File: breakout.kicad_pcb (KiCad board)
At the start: 2 copper layers, 20.7 x 16.1 mm, 7 parts, among them J1 Conn_01x03, J2 Conn_01x02

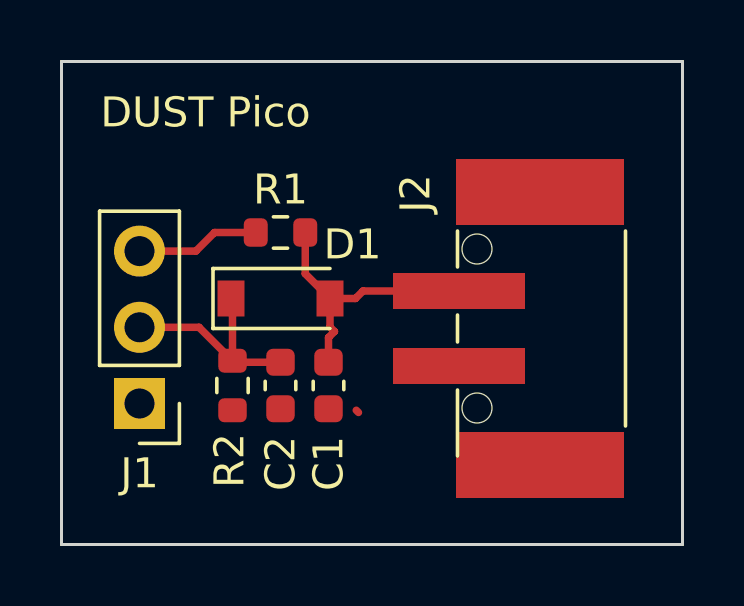
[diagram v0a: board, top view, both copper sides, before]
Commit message: v1.0
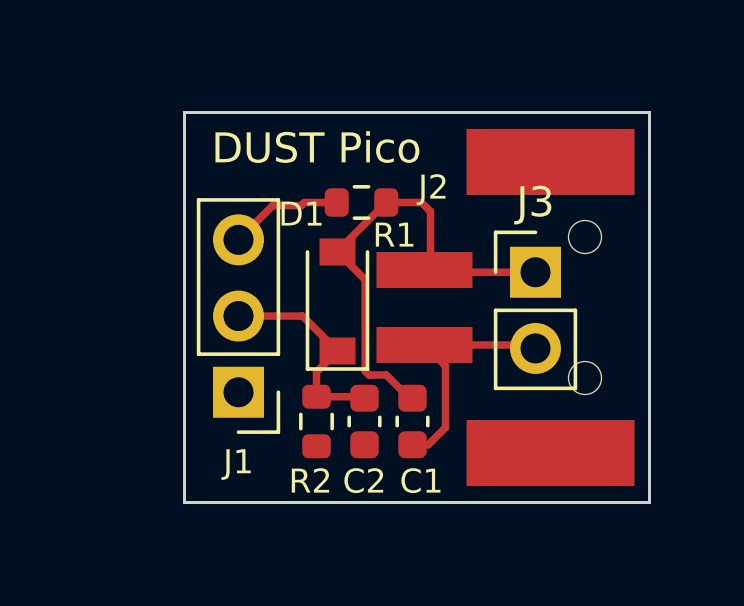
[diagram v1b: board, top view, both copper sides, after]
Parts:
- added J3: Conn_01x02, Connector_PinHeader_2.54mm:PinHeader_1x02_P2.54mm_Vertical, F.Cu at (152.2, 76.3)
- J2: footprint TerminalBlock_Phoenix:TerminalBlock_Phoenix_PTSM-0,5-2-HV-2.5-SMD_1x02-1MP_P2.50mm_Vertical -> DUST:PTSM 0.5-2-HH-2.5-SMD
- moved J1 3.32 mm to (142.3, 80.3)
- moved C2 3.05 mm to (146.5, 81.3)
- moved R2 3.05 mm to (144.9, 81.3)
- moved C1 3.05 mm to (148.1, 81.3)
- moved R1 2.88 mm to (146.4, 74.0)
- moved D1 1.90 mm to (145.6, 77.3), turned to 90 degrees
- moved J2 1.00 mm to (151.6, 77.2), turned to 90 degrees
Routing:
- net Net-(C1-Pad1): track 9.22 -> 16.0 mm
- net GND: track 1.91 -> 8.13 mm
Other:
- board size 20.7 x 16.1 mm -> 15.5 x 13 mm
- board text added: "SENS"
- board text added: "Sille Van Landschoot Nico De Witte"
- board text added: "V1.0 - 2021"
